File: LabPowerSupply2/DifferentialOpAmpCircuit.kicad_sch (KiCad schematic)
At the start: 14 parts

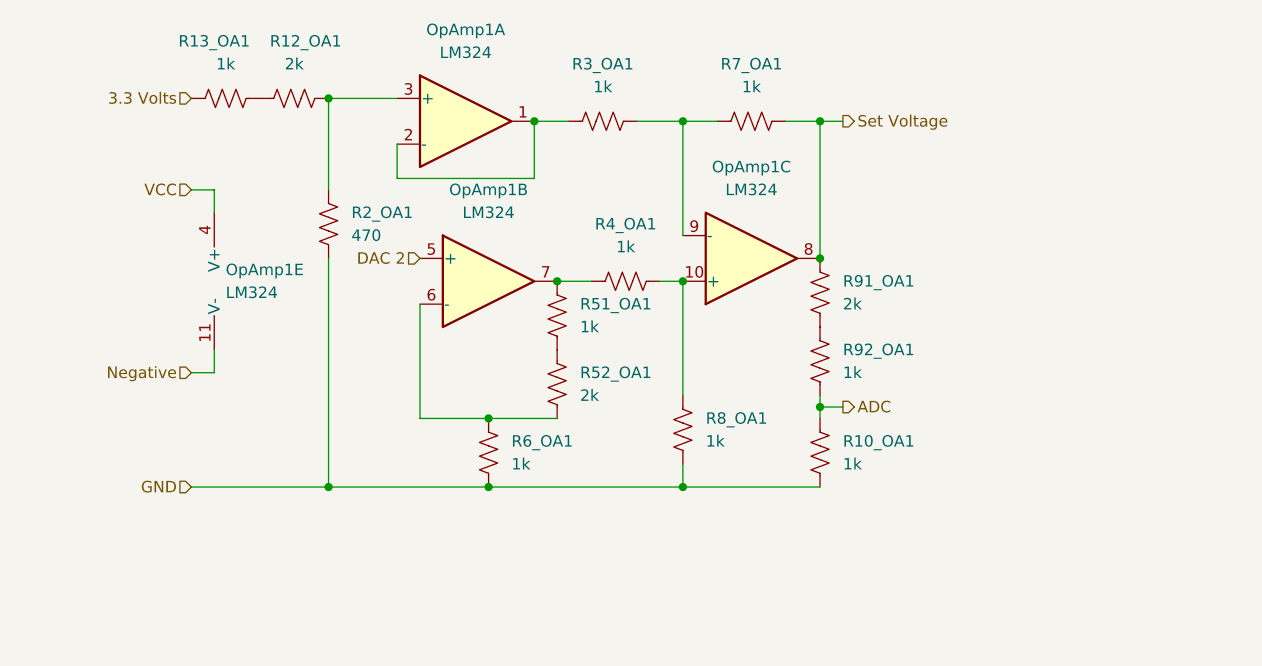
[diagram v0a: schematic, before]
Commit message: Beautifing the Schematic
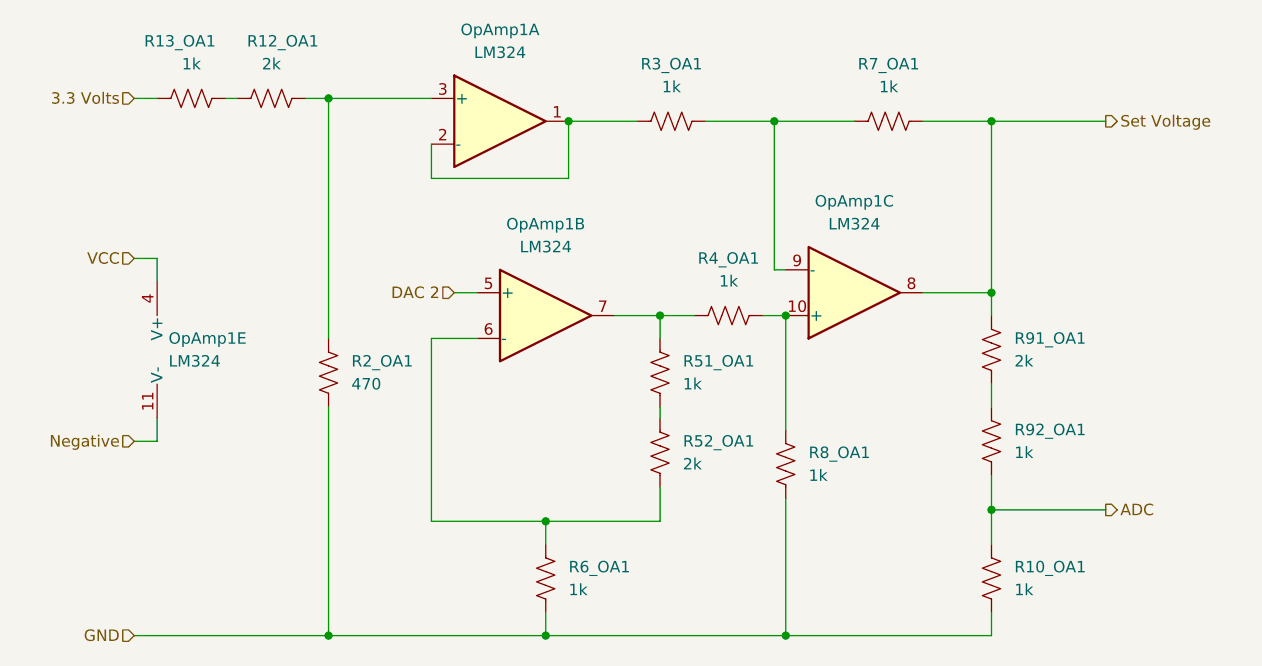
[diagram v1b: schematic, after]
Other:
- moved on the sheet: OpAmp1A, OpAmp1B, OpAmp1C, OpAmp1E, R10_OA1, R12_OA1, R13_OA1, R2_OA1, R3_OA1, R4_OA1, R51_OA1, R52_OA1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
